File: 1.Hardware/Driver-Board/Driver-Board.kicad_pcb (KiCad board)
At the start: 4 copper layers, 42.3 x 42.3 mm, 75 parts, among them J1 Conn_01x04, J2 Conn_01x02, J3 Conn_01x02, J4 Conn_01x04, J5 Conn_01x02, J6 Conn_01x02, Q1 FDN352AP, SW1 SW_Push, U1 MP2456, U2 MCP1700-3302E_SOT23, U3 TJA1051T-3, U4 AS5600, U5 TB67H450FNG,EL, U6 TB67H450FNG,EL, U7 STM32F103C6Tx, Y1 12MHz

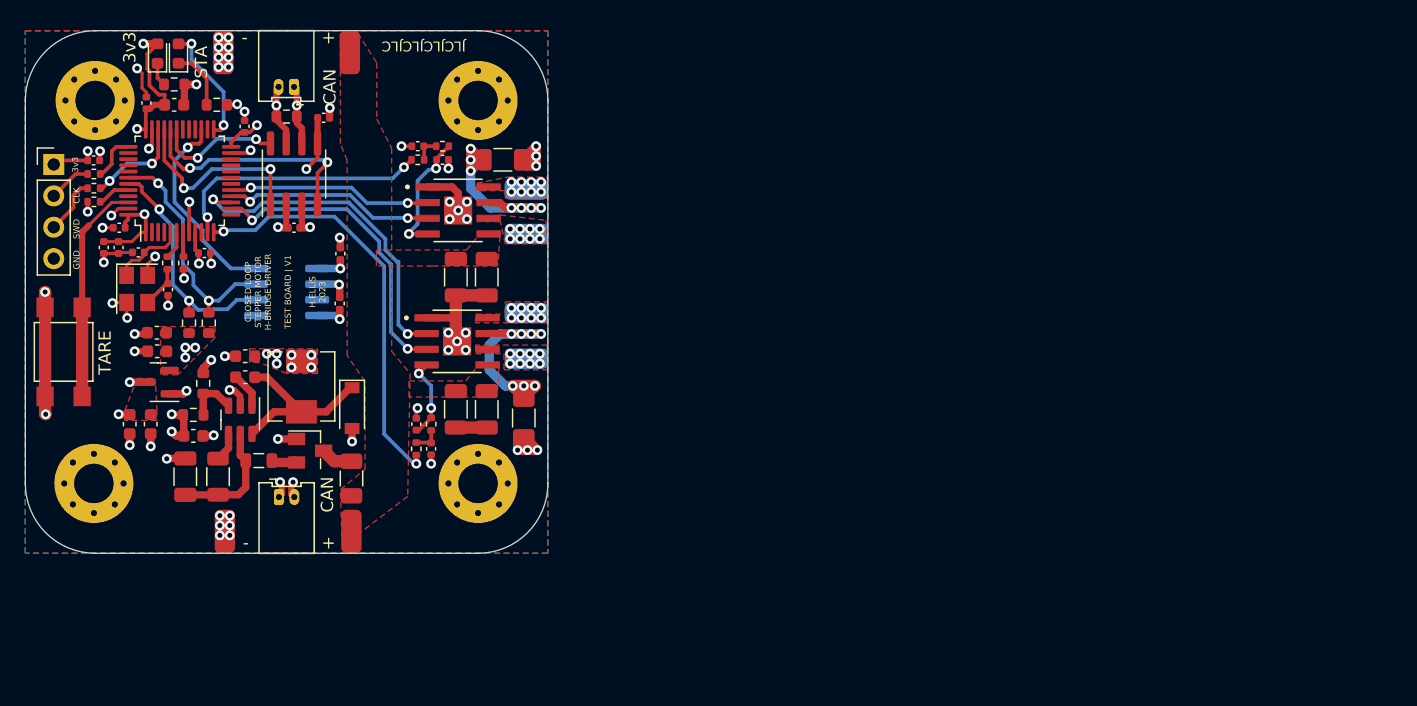
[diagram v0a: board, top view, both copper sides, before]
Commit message: updated board
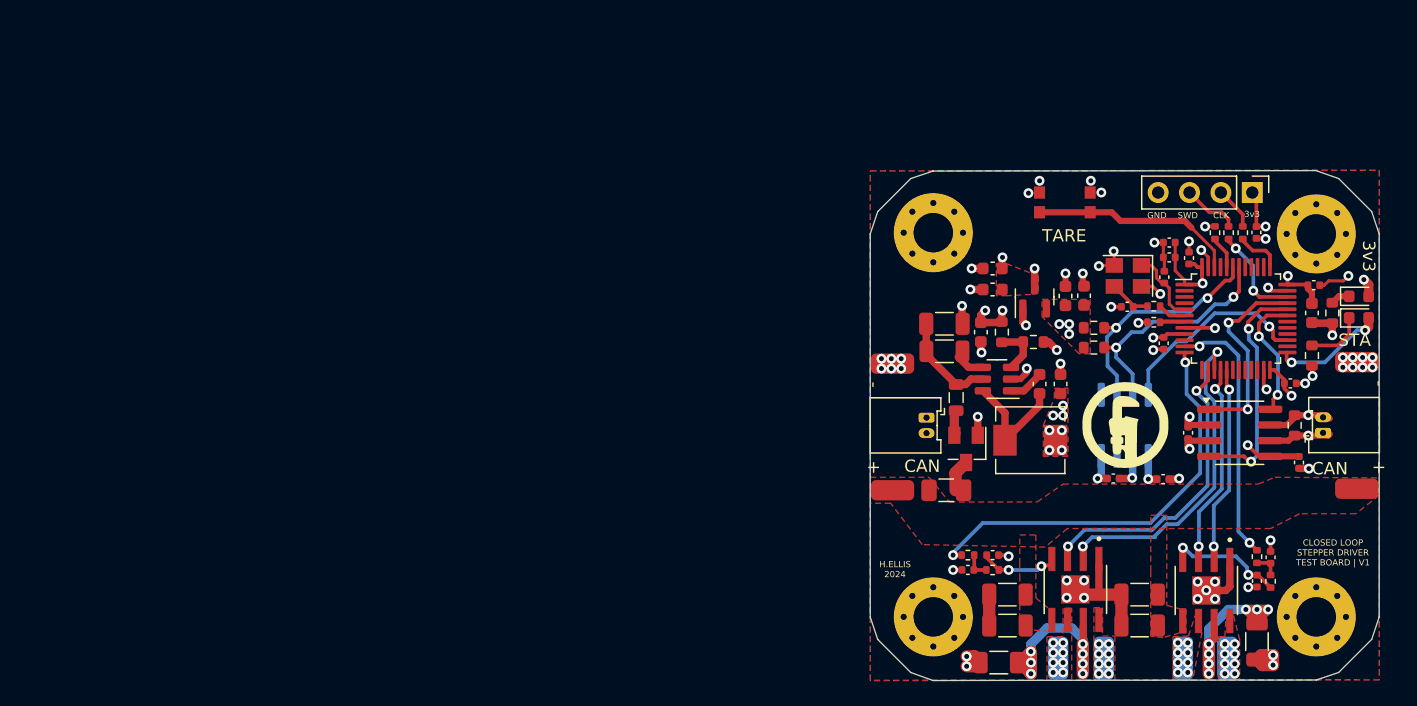
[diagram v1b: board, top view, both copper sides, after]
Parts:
- removed D1: B5819W, Diode_SMD:D_SOD-123
- added G***: LOGO, LOGO, F.Cu at (150.0, 100.3)
- L1: value L_Small -> 22uH
- SW1: footprint Button_Switch_SMD:SW_SPST_TL3305B -> custom:KMR731NG LFS
- moved H3 99.4 mm to (165.4, 84.9), turned to -90 degrees
- moved D2 99.2 mm to (168.9, 90.0), turned to 0 degrees
- moved D3 97.9 mm to (168.9, 91.7), turned to 0 degrees
- moved J1 97.0 mm to (160.3, 81.5), turned to -90 degrees
- moved C14 95.6 mm to (165.2, 89.0), turned to 0 degrees
- moved R8 95.6 mm to (166.8, 91.3), turned to -90 degrees
- moved C6 94.3 mm to (160.6, 84.8), turned to -90 degrees
- moved J6 94.0 mm to (170.5, 100.3), turned to 90 degrees
- moved C12 93.6 mm to (165.1, 91.3), turned to -90 degrees
- moved R4 93.1 mm to (159.5, 84.8), turned to 90 degrees
- moved R5 91.9 mm to (158.3, 84.8), turned to 90 degrees
- moved R19 90.9 mm to (165.1, 94.8), turned to -90 degrees
- moved R12 90.8 mm to (157.2, 84.8), turned to -90 degrees
- moved J3 87.9 mm to (166.0, 101.0), turned to 90 degrees
- moved C15 87.2 mm to (163.3, 97.0), turned to 0 degrees
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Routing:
- net GND: track 89.7 -> 72.7 mm, vias 69 -> 67
- net +3.3V: track 60.3 -> 53.9 mm
- net BUCK_SW: track 14.6 -> 9.68 mm
- net CAN-: track 44.6 -> 41.9 mm, vias 2 -> 1
- net CAN+: track 45.0 -> 42.7 mm, vias 2 -> 1
- net BUCK_IN: track 9.83 -> 8.26 mm
- net BUTTON: track 18.8 -> 17.5 mm
- net Net-(U5-RS): track 23.6 -> 24.7 mm
- net Net-(U6-RS): track 19.7 -> 18.7 mm
- net CAN_RX: track 19.5 -> 18.8 mm
- net LED: track 9.84 -> 9.25 mm
- net A_CURRENT: track 6.57 -> 6.05 mm
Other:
- board size 42.3 x 42.3 mm -> 41.2 x 41.3 mm
- board text added: "CLOSED LOOP STEPPER DRIVER TEST BOARD | V1"
- board text added: "H.ELLIS 2024"
- board text removed: "CLOSED LOOP STEPPER MOTOR H-BRIDGE DRIVER TEST BOARD | V1"
- board text removed: "H.ELLIS 2023"
- board text removed: "JLCJLCJLCJLC"
